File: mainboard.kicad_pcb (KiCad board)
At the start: 2 copper layers, 157.6 x 135.8 mm, 57 parts, among them J1 DRV8833-1, J13 Conn_PCA9685, J14 Conn_01x02, J15 Conn_01x02, J16 Conn_01x02, J18 Screw_Terminal_01x06, J19 Screw_Terminal_01x06, J2 DRV8833-0, J20 Screw_Terminal_01x06, J21 Screw_Terminal_01x06, J22 Screw_Terminal_01x06, J23 Screw_Terminal_01x06, J24 Screw_Terminal_01x04, J25 Screw_Terminal_01x02, J27 Rotary Encoder Conn, J28 Conn_01x02, J3 Conn_01x02, J4 Screw_Terminal_01x06, J5 Screw_Terminal_01x06, J6 VIM4_HEADER, J7 Screw_Terminal_01x06, J8 Screw_Terminal_01x06, Q3 2N7000, Q4 2N7000, U1 MCP23017_SP

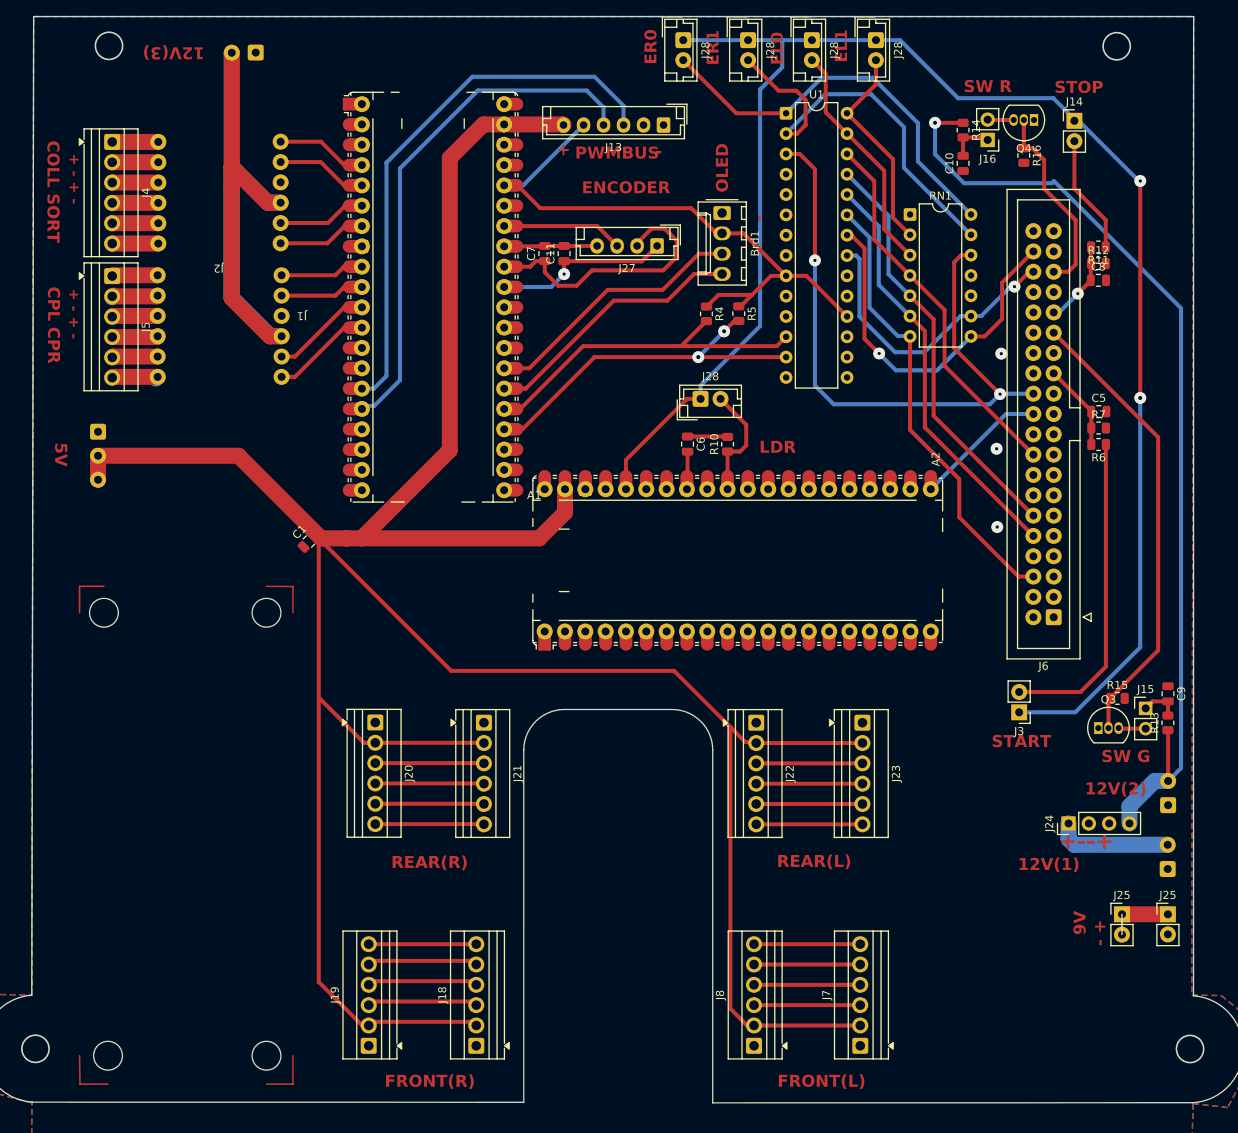
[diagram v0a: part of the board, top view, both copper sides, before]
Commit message: V1.2
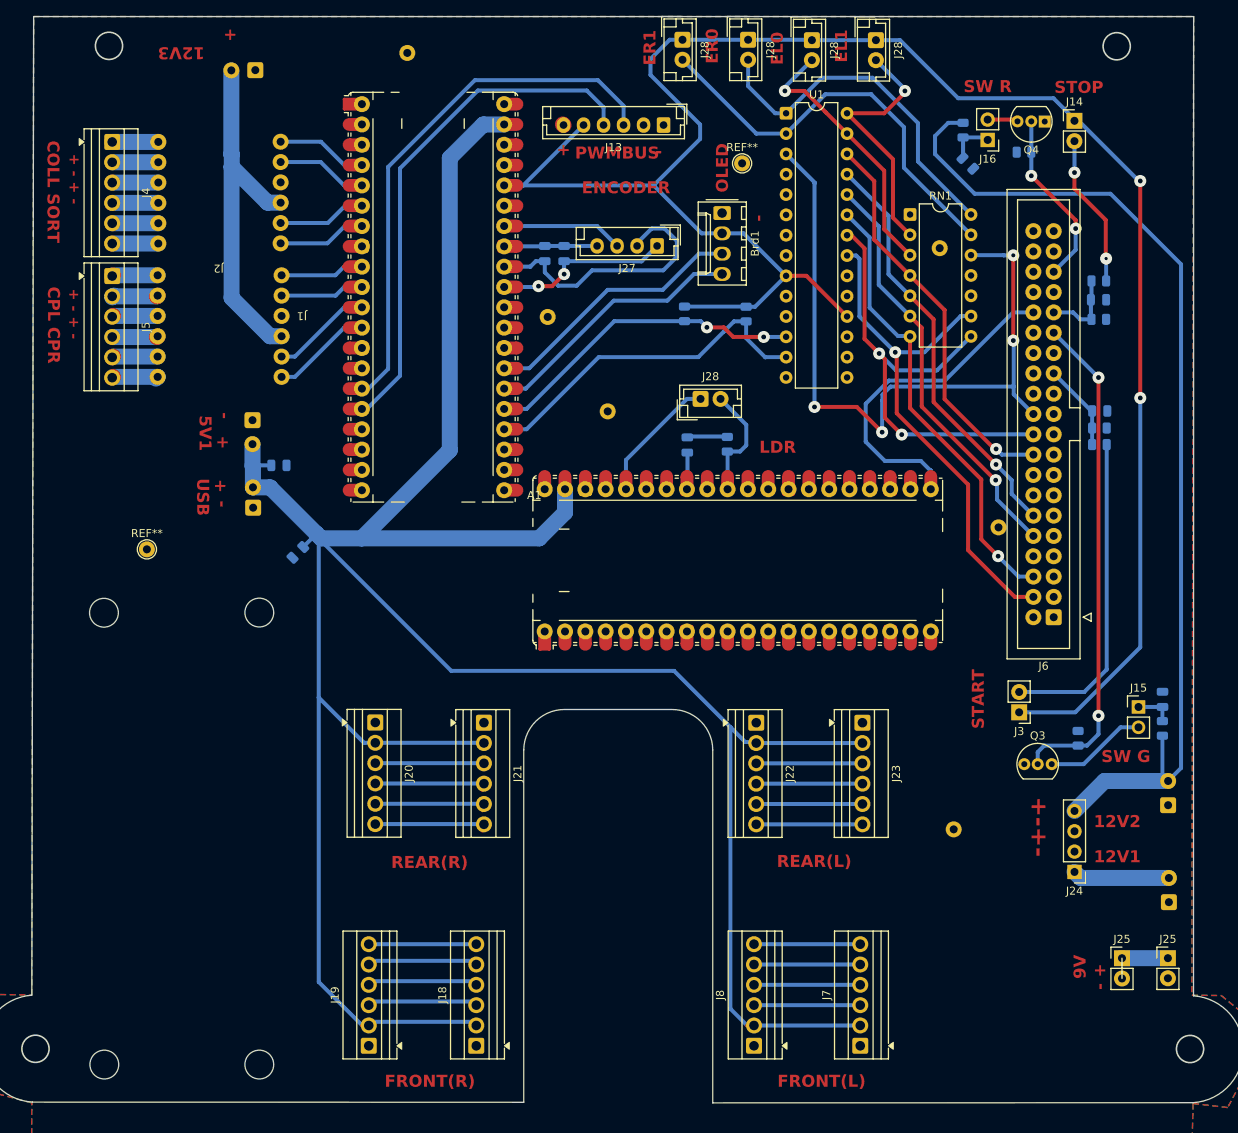
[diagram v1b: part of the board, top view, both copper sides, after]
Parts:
- added ?: , clipboard:9c2f8d19-4101-4f98-a26c-8554f3c2bdce, F.Cu at (289.9, 91.8)
- added ?: , , F.Cu at (334.2, 82.3)
- added ?: , , F.Cu at (377.5, 134.6)
- added ?: , , F.Cu at (309.2, 37.5)
- added ?: , , F.Cu at (326.7, 70.5)
- added ?: , , F.Cu at (383.1, 96.8)
- added ?: , , F.Cu at (375.7, 61.9)
- added C1: 1uF, Capacitor_SMD:C_0805_2012Metric, B.Cu at (293.1, 89.1)
- added REF**: TestPoint_THTPad_D2.0mm_Drill1.0mm, TestPoint:TestPoint_THTPad_D2.0mm_Drill1.0mm, F.Cu at (351.0, 51.3)
- added REF**: TestPoint_THTPad_D2.0mm_Drill1.0mm, TestPoint:TestPoint_THTPad_D2.0mm_Drill1.0mm, F.Cu at (276.6, 99.6)
- C1, C10, C11, C5, C6, C7, C8, C9, R10, R11, R12, R13, R14, R15, R16, R4, R5, R6, R7: moved to B.Cu
- moved ? 19.4 mm to (289.8, 86.4)
- moved Q3 9.93 mm to (386.7, 126.4)
- moved J28 8.20 mm to (343.6, 35.9)
- moved J28 8.10 mm to (351.8, 35.9)
- moved R15 7.00 mm to (393.0, 123.2), turned to 90 degrees
- moved R12 6.96 mm to (395.6, 70.8)
- moved J24 6.10 mm to (392.6, 139.9), turned to 180 degrees
- moved J25 5.48 mm to (398.5, 150.7)
- moved J25 5.48 mm to (404.3, 150.7)
- moved R11 4.25 mm to (395.6, 66.0)
- moved ? 4.15 mm to (404.4, 140.6)
- moved R4 2.74 mm to (343.8, 70.1)
- moved C8 2.43 mm to (395.6, 68.4)
- moved ? 2.20 mm to (287.2, 39.7)
- moved C1 1.93 mm to (295.5, 99.9)
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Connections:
- J13 pad 6: 5V_BUCK -> 5V_BUCK2
- J14 pad 1: PICO2_3V3 -> PICO1_3V3
- J28 pad 1: PICO2_3V3 -> PICO1_3V3 (x4)
- J3 pad 1: PICO2_3V3 -> PICO1_3V3
- J6 pad 22: unconnected-(J6-Pin_22-Pad22) -> COLL(en/dis)
- J6 pad 30: unconnected-(J6-Pin_30-Pad30) -> SORT(en/dis)
- J6 pad 31: PIC_STATE -> TOTEM-EXTEND
- J6 pad 32: TOTEM-EXTEND -> unconnected-(J6-Pin_32-Pad32)
- J6 pad 33: BOOM(ext/ret) -> unconnected-(J6-Pin_33-Pad33)
- J6 pad 36: unconnected-(J6-Pin_36-Pad36) -> PIC_STATE
- J6 pad 38: COLL(en/dis) -> unconnected-(J6-Pin_38-Pad38)
- J6 pad 39: SORT(en/dis) -> unconnected-(J6-Pin_39-Pad39)
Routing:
- net PICO2_3V3: track 205.9 -> 15.3 mm, vias 2 -> 0
- net PICO1_3V3: track 75.7 -> 246.0 mm, vias 0 -> 2
- net 12V_BUCK3: track 93.8 -> 44.7 mm
- net COLL(en/dis): track 36.8 -> 65.8 mm
- net PIC_STATE: track 16.7 -> 42.4 mm
- net 5V_BUCK: track 368.8 -> 348.2 mm
- net SORT(en/dis): track 45.9 -> 58.8 mm, vias 1 -> 2
- net Net-(J15-Pin_2): track 3.41 -> 12.8 mm
- net TOTEM-EXTEND: track 81.6 -> 90.7 mm, vias 2 -> 4
- net 12V_BUCK2: track 120.8 -> 127.4 mm, vias 1 -> 0
- net CP-R-ENDSTOP0: track 50.4 -> 44.3 mm
- net CP-L-ENDSTOP1: track 26.7 -> 32.5 mm, vias 0 -> 1
- net GREEN: track 57.4 -> 62.5 mm, vias 0 -> 2
- net CP-L-ENDSTOP0: track 29.5 -> 33.7 mm, vias 0 -> 1
- net Net-(J14-Pin_2): track 15.1 -> 19.1 mm, vias 0 -> 2
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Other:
- outline, holes or cut-outs redrawn
- board text added: "+-+-"
- board text added: "12V1"
- board text added: "12V2"
- board text added: "12V3"
- board text added: "5V1"
- board text added: "USB"
- board text removed: "+--+"
- board text removed: "12V(1)"
- board text removed: "12V(2)"
- board text removed: "12V(3)"
- board text removed: "5V"
